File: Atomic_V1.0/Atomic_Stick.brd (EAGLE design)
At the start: 14 parts, among them U4 TLE9250VSJ

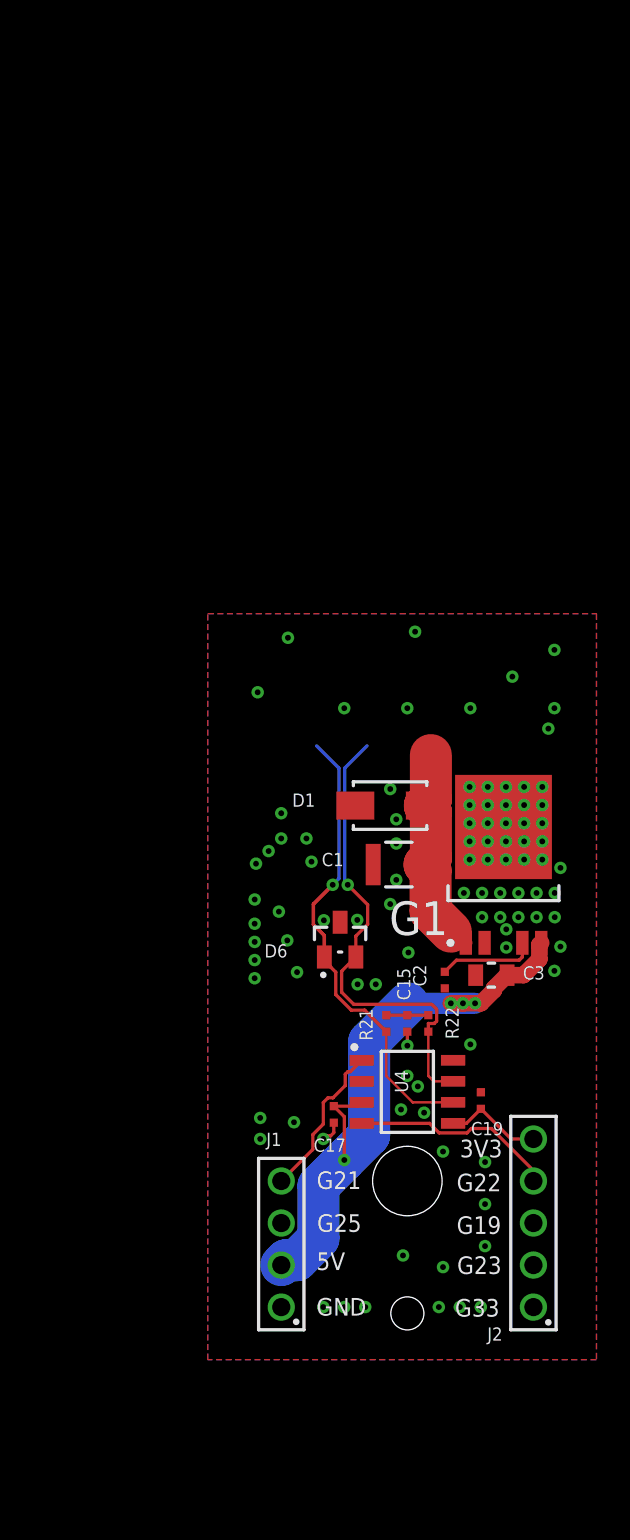
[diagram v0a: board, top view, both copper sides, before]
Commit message: ..
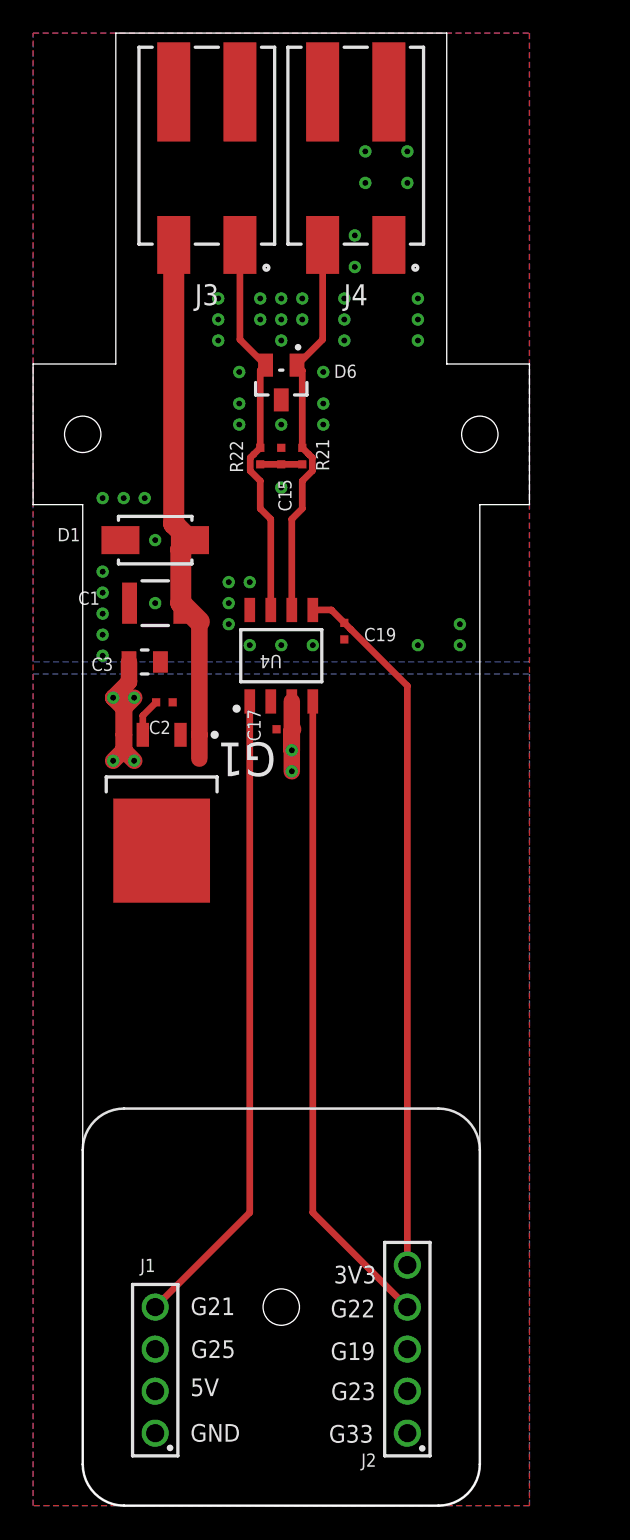
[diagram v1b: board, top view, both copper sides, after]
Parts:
- added J3, J4: (no value), Wurth_Connectors_WR-LECO:695402400222
- moved R22 35.8 mm to (-1.27, 51.4), turned to 270 degrees
- moved C15 35.1 mm to (0.00, 51.4), turned to 90 degrees
- moved R21 34.7 mm to (1.27, 51.4), turned to 90 degrees
- moved D6 33.9 mm to (0.00, 55.9), turned to 270 degrees
- moved C19 29.5 mm to (3.81, 40.9), turned to 270 degrees
- moved C3 28.2 mm to (-8.25, 39.0), turned to 180 degrees
- moved U4 27.4 mm to (0.00, 39.4), turned to 90 degrees
- moved C2 23.9 mm to (-7.06, 36.6), turned to 0 degrees
- moved C17 23.5 mm to (0.21, 34.9), turned to 180 degrees
- moved C1 21.6 mm to (-7.62, 42.5)
- moved D1 21.4 mm to (-7.62, 46.4)
- moved G1 20.9 mm to (-7.23, 29.9), turned to 270 degrees
- moved J1 10.8 mm to (-7.62, -3.81)
- moved J2 10.8 mm to (7.62, -2.54)
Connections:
- net +12V: now also J3.2, J3.A2
- net CAN_H: now also J3.1, J3.A1
- net CAN_L: now also J4.2, J4.A2
- net GND: now also J4.1, J4.A1
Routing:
- net +3V3: track 5.98 -> 42.6 mm
- net CAN1_TXD: track 9.57 -> 39.0 mm
- net CAN1_RXD: track 12.4 -> 39.0 mm
- net +5V: track 37.0 -> 16.8 mm, vias 4 -> 6
- net +12V: track 13.0 -> 32.1 mm
- net CAN_L: track 33.2 -> 23.6 mm, vias 1 -> 0
- net CAN_H: track 28.9 -> 23.6 mm, vias 1 -> 0
- net N$1: track 5.92 -> 2.30 mm
- net GND: track 2.43 -> 0.00 mm, vias 97 -> 50
- added copper zone on layer 16, net +5V
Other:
- board outline added: 30 x 89 mm
